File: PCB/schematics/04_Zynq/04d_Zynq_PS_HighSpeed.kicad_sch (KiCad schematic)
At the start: 36 parts, among them CN1 1-2199230-6, U39 TPD4E05U06DQA, Y3 SiT9365AI-4B2-33E100.0000000

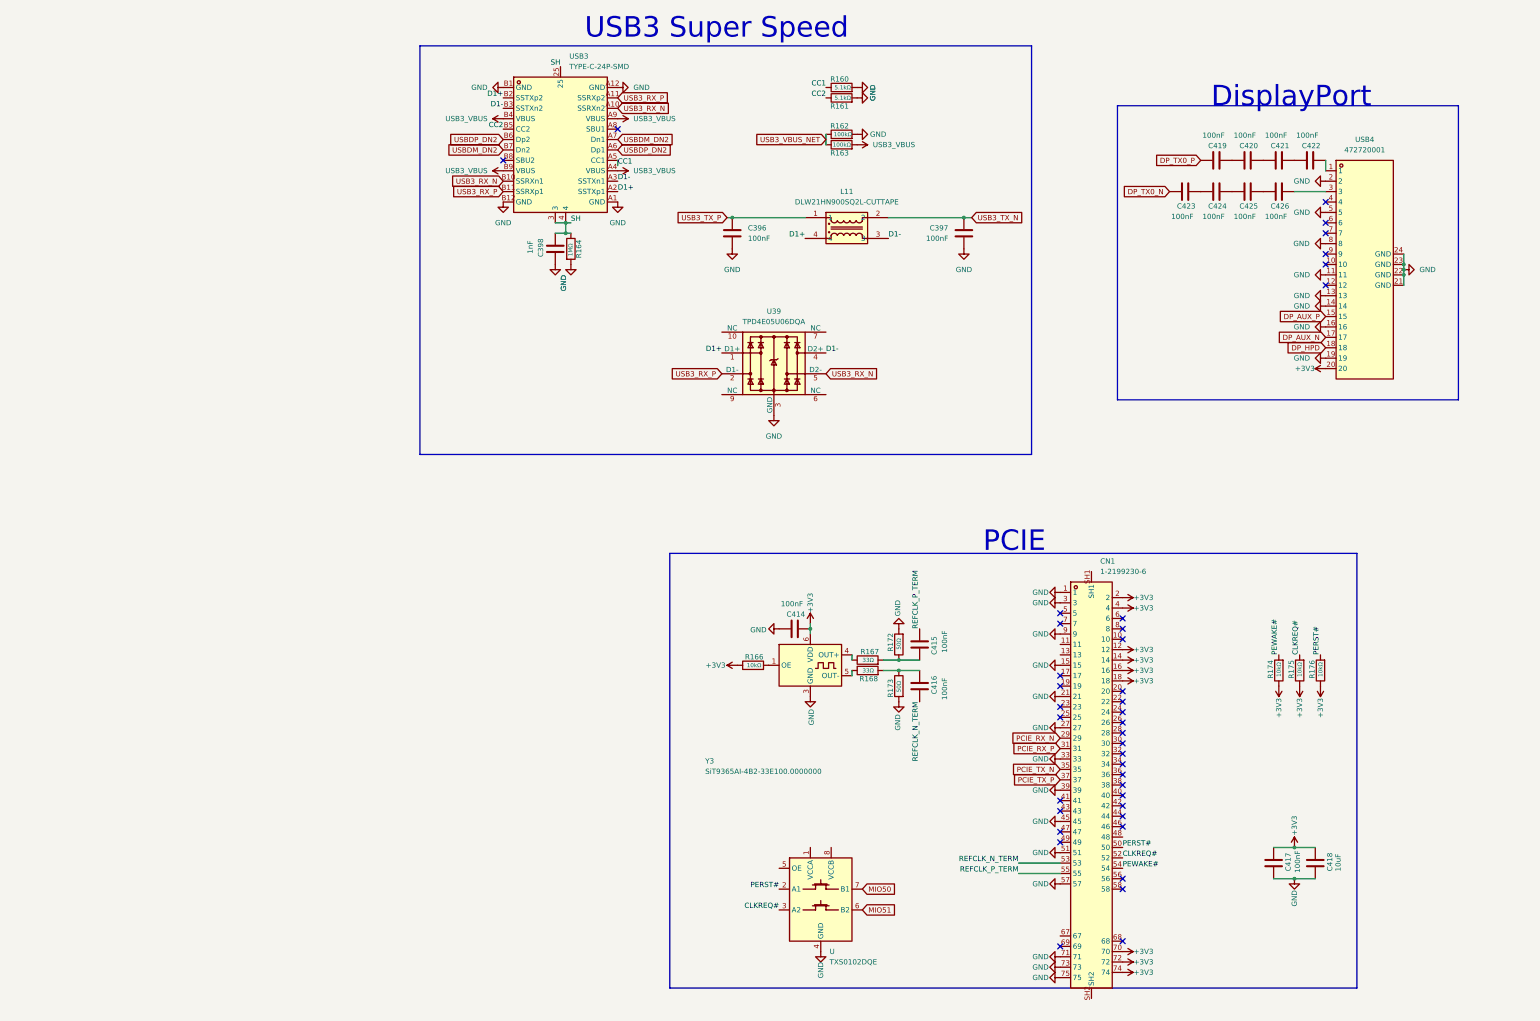
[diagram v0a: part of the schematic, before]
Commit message: Feat : Schematics Complete
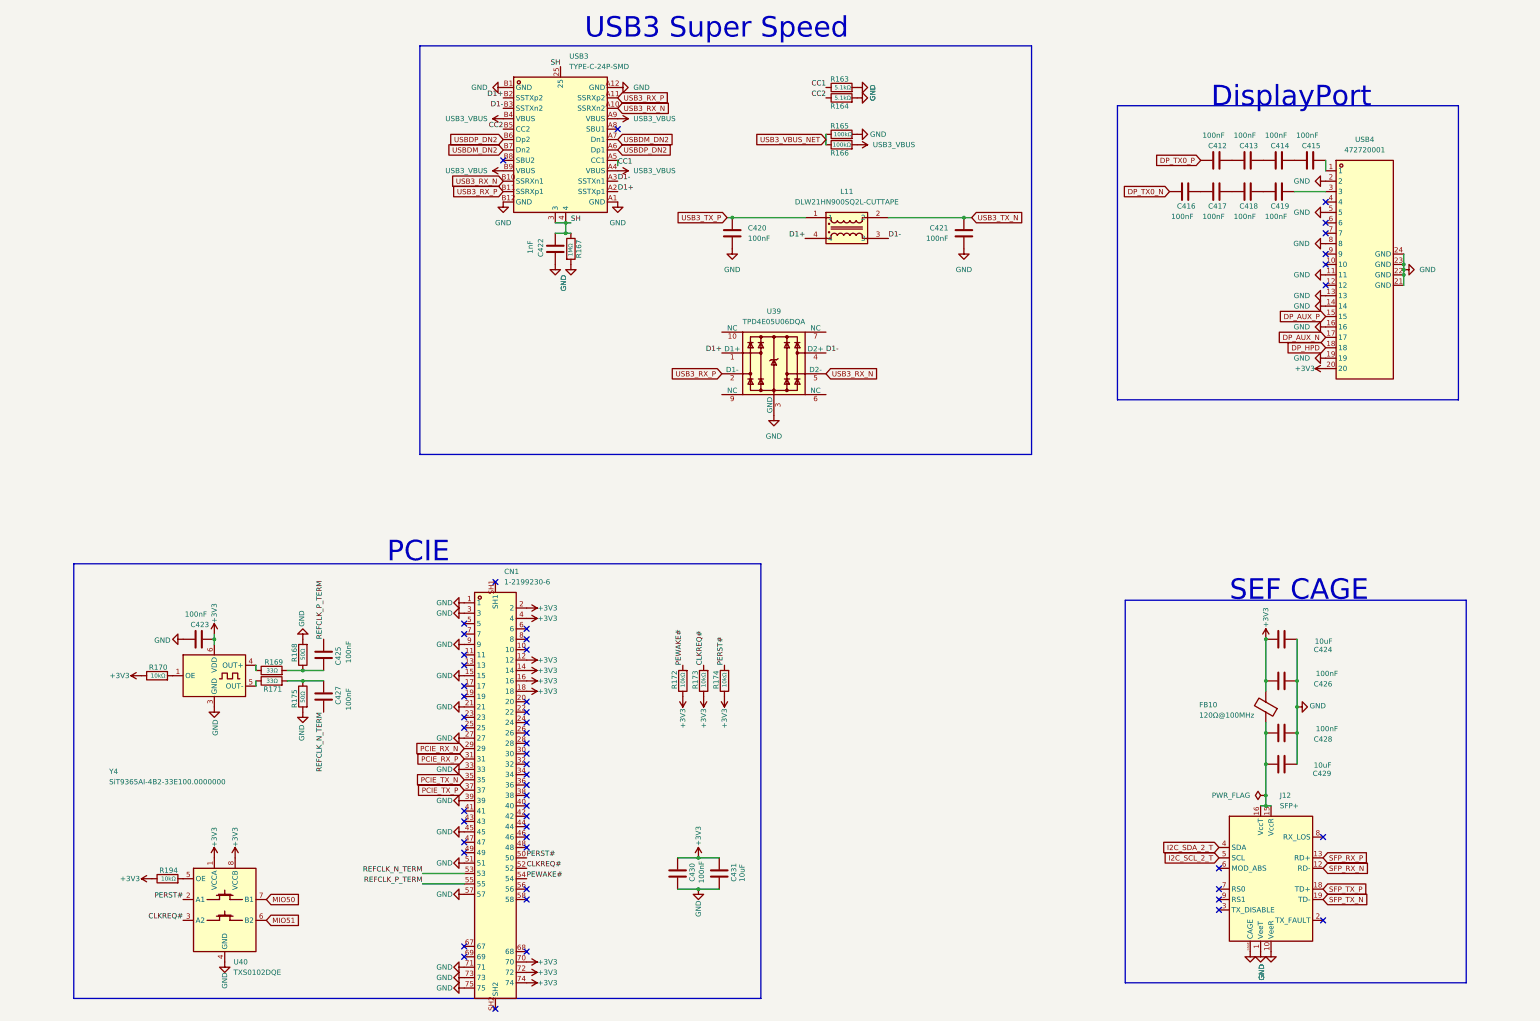
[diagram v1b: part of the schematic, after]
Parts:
- added C424, C429: 10uF, Capacitor_SMD:C_0805_2012Metric, symbol Device:C
- added C426, C428: 100nF, Capacitor_SMD:C_0402_1005Metric, symbol Device:C
- added FB10: 120Ω@100MHz, Inductor_SMD:L_01005_0402Metric, symbol Device:FerriteBead
- added J12: SFP+, Connector:Connector_SFP_and_Cage, symbol Interface_Optical:SFP+
- added R194: 10kΩ, Resistor_SMD:R_0402_1005Metric, symbol Device:R
- renumbered C419 to C412, C420 to C413, C421 to C414, C422 to C415, C423 to C416, C424 to C417, C425 to C418, C426 to C419, C396 to C420, C397 to C421, C398 to C422, C414 to C423, C415 to C425, C416 to C427, C417 to C430, C418 to C431, R160 to R163, R161 to R164, R162 to R165, R163 to R166, R164 to R167, R172 to R168, R167 to R169, R166 to R170, R168 to R171, R174 to R172, R175 to R173, R176 to R174, R173 to R175, U to U40, Y3 to Y4
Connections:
- net +3V3: now also U40.1 (VCCA), U40.8 (VCCB), C424.2, C426.2, FB10.2, R194.1
- net GND: now also C424.1, C426.1, C428.1, C429.1, J12.1 (VeeT), J12.10 (VeeR), J12.11 (VeeR), J12.14 (VeeR), J12.17 (VeeT), J12.20 (VeeT), J12.CAGE
- net at U40.5 (OE): now also R194.2
- new net: C428.2, C429.2, FB10.1, J12.15 (VccR), J12.16 (VccT)
- new net I2C_SCL_2_T: J12.5 (SCL)
- new net I2C_SDA_2_T: J12.4 (SDA)
- new net SFP_RX_N: J12.12 (RD-)
- new net SFP_RX_P: J12.13 (RD+)
- new net SFP_TX_N: J12.19 (TD-)
- new net SFP_TX_P: J12.18 (TD+)
- no-connect marks 39 -> 51
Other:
- note added: "SEF CAGE"
- moved on the sheet: C423, C425, C427, C430, C431, CN1, R168, R169, R170, R171, R172, R173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
